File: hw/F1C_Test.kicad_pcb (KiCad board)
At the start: 2 copper layers, 32 x 56 mm, 66 parts, among them J1 USB_C_Receptacle_USB2.0_14P, J2 FPC/FFC P0.5, J3 1x03 P2.54, J4 1x06 P2.54, J5 AudioJack4, SW1 SW_Push, SW2 SW_Push, SW3 SW_SPST, U1 ME3103, U2 ME3103, U3 ME3103, U4 F1C100s, U5 W25Q32JVSS, U6 MT9284, Y1 24MHz 20pF

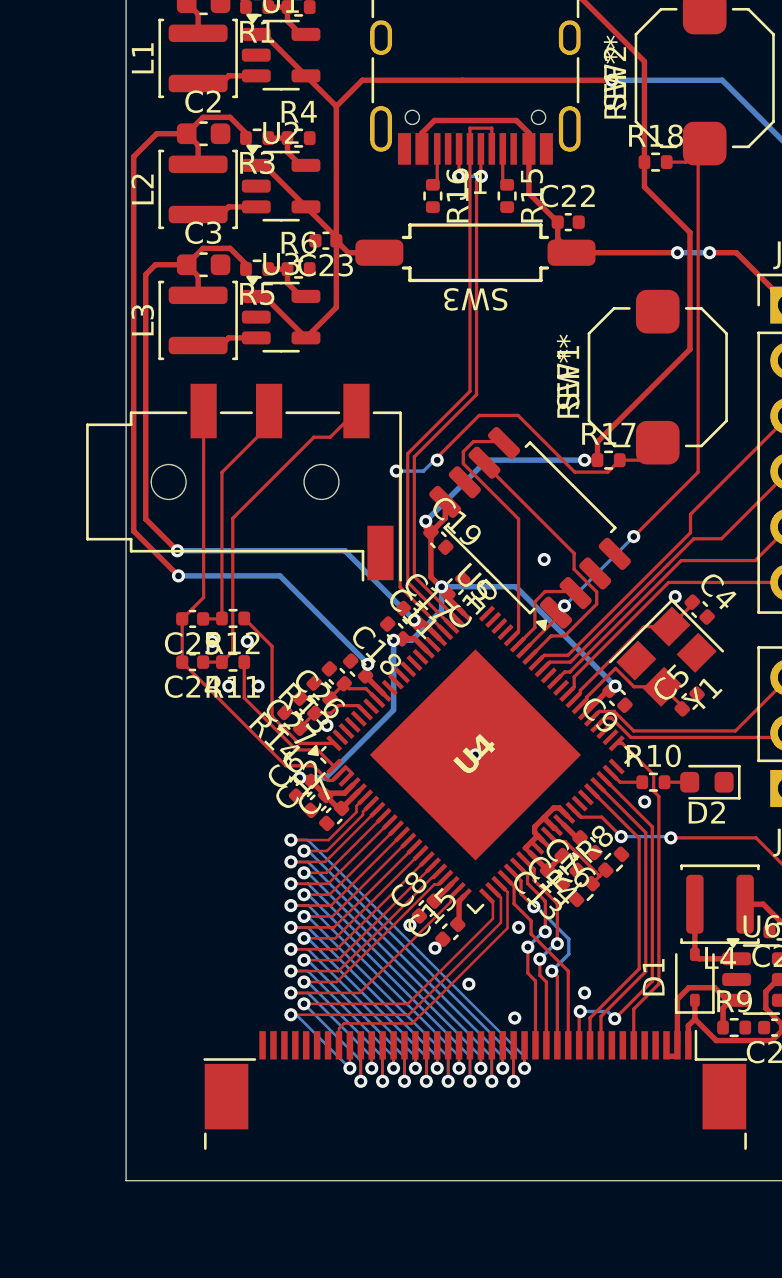
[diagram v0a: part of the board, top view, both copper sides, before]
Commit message: hw: Finish routing, finally
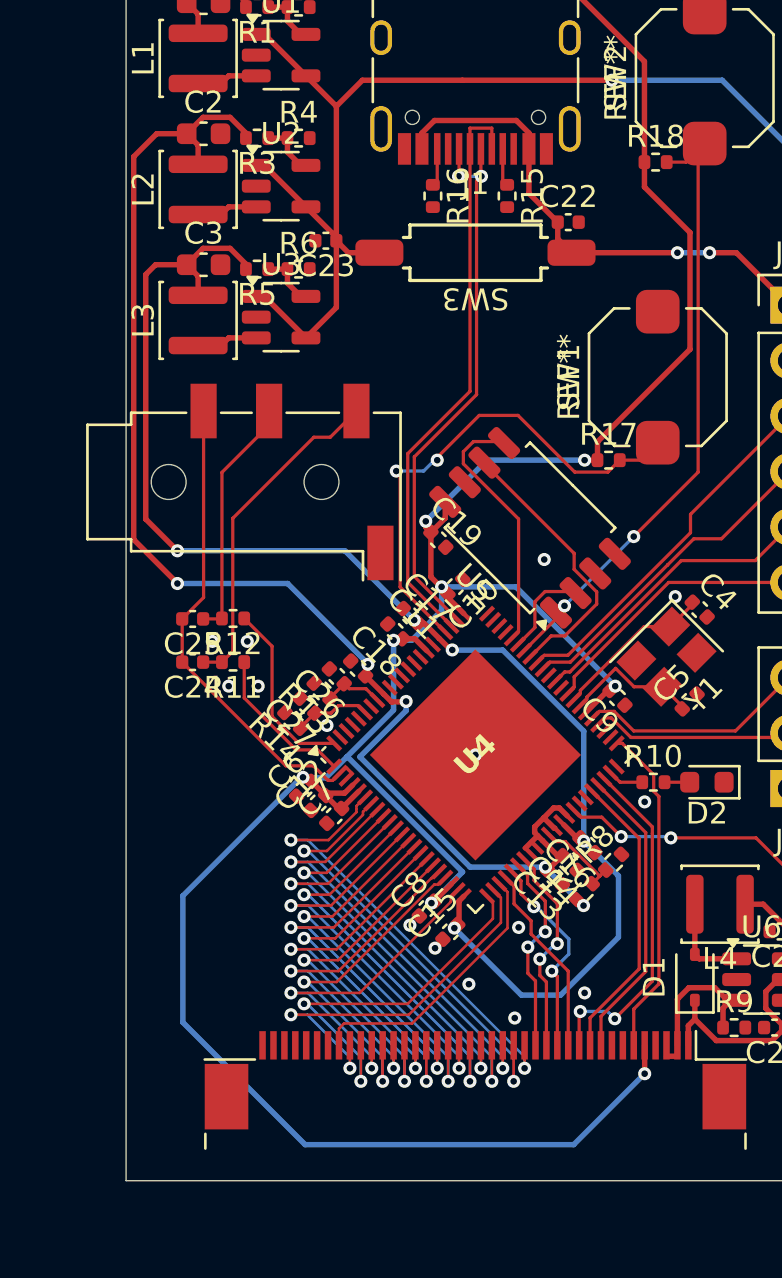
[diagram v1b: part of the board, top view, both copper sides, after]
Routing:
- net +3V3: track 94.4 -> 143.5 mm, vias 6 -> 8
- net +1V1: track 36.5 -> 65.4 mm, vias 2 -> 5
- net +2V6: track 46.6 -> 65.0 mm, vias 2 -> 5
